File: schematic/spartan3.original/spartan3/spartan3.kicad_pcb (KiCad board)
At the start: 2 copper layers, 214.6 x 160 mm, 240 parts, among them U1_clk_select_0 SPFT_Sliding_Switch-dynacore, U2 XC3S250E-4TQG144C

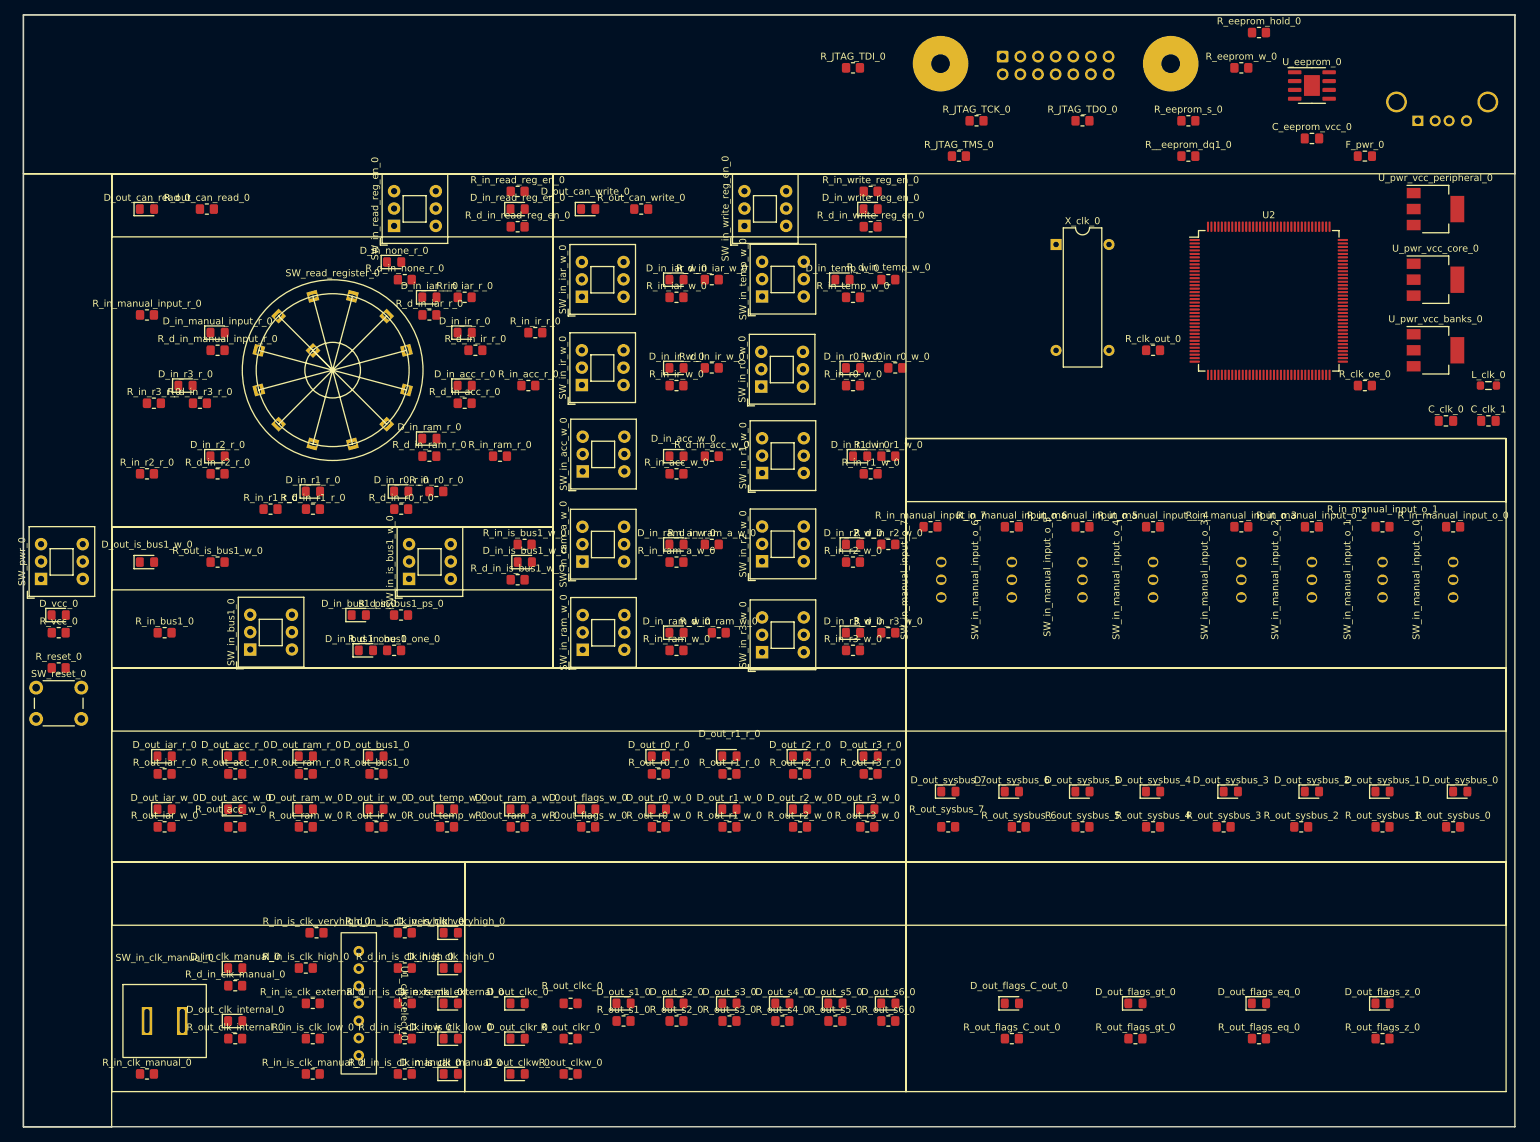
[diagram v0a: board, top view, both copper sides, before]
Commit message: PCB layout :: updated
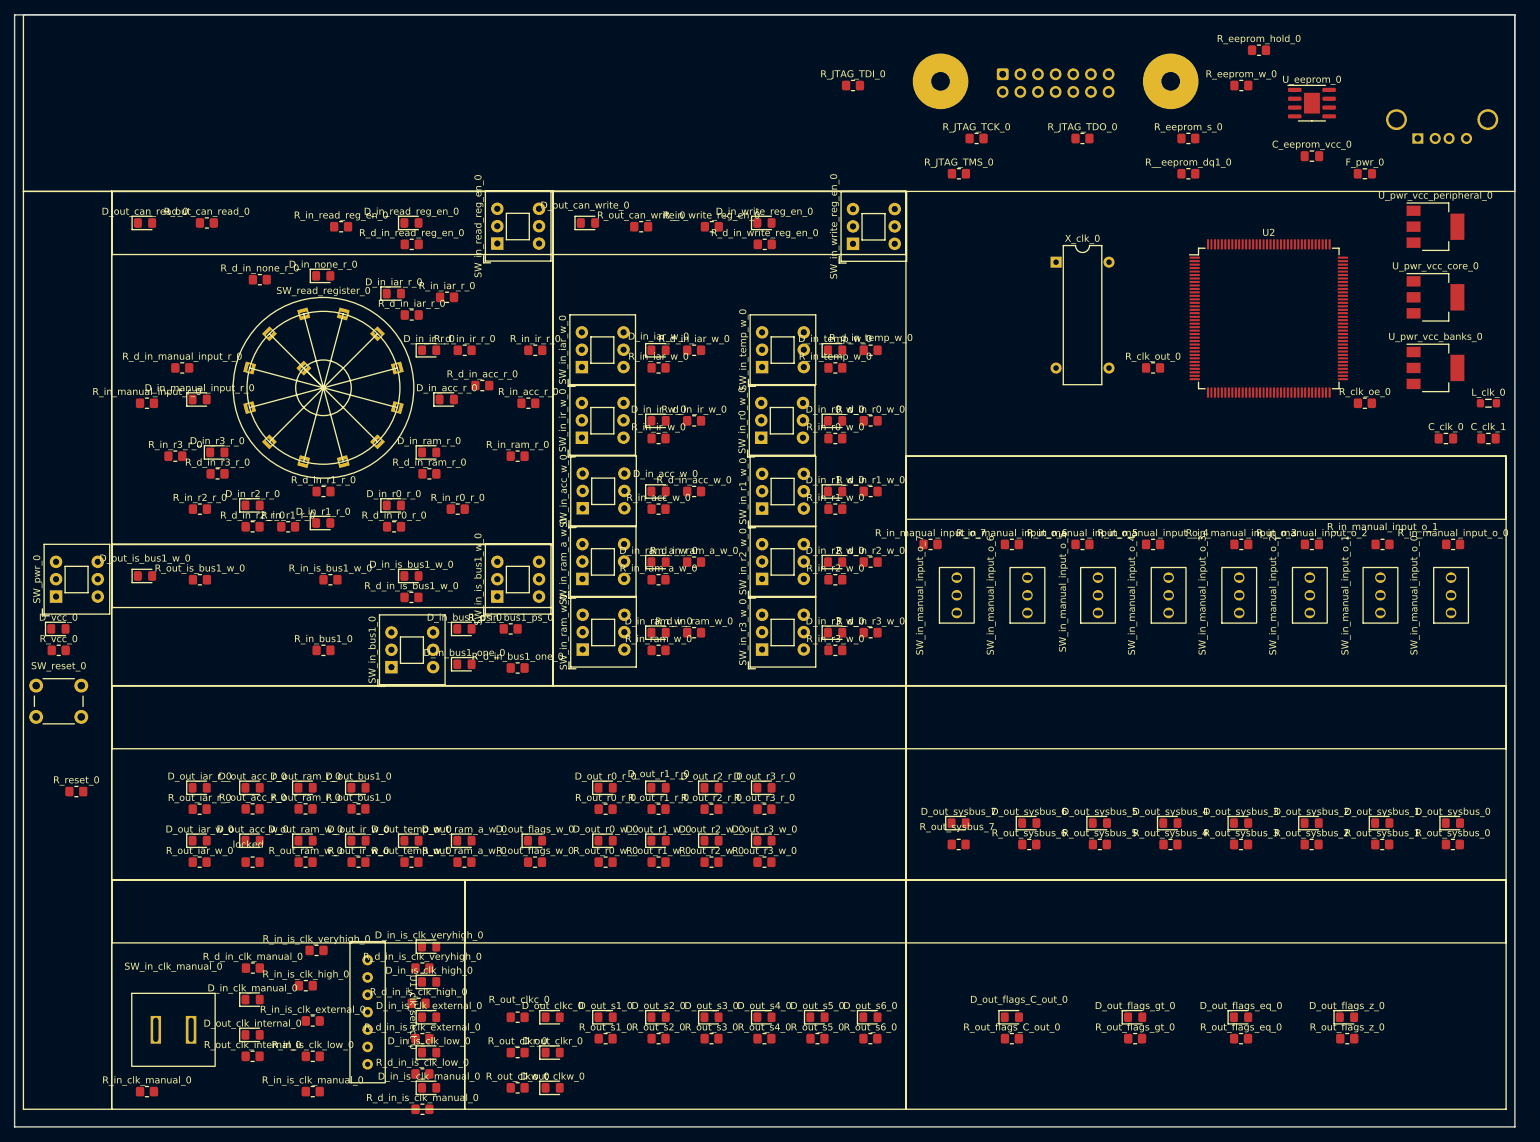
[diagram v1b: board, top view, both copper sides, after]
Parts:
- moved R_in_is_bus1_w_0 28.4 mm to (44.2, 81.3)
- moved R_in_read_reg_en_0 25.9 mm to (45.7, 30.5)
- moved R_in_write_reg_en_0 23.4 mm to (99.1, 30.5)
- moved R_in_bus1_0 23.0 mm to (43.2, 91.4)
- moved R_d_in_none_r_0 20.9 mm to (34.0, 38.1)
- moved SW_in_bus1_0 20.5 mm to (53.0, 93.9)
- moved R_d_in_bus1_one_0 18.0 mm to (71.1, 94.0)
- moved R_reset_0 18.0 mm to (7.62, 111.8)
- moved D_in_is_bus1_w_0 16.4 mm to (55.8, 80.7)
- moved R_out_r3_r_0 16.1 mm to (106.6, 114.3)
- moved D_out_r3_r_0 15.9 mm to (106.6, 111.2)
- moved R_d_in_bus1_ps_0 15.9 mm to (70.1, 88.4)
- moved SW_in_write_reg_en_0 15.8 mm to (119.4, 32.9)
- moved R_out_r3_w_0 15.6 mm to (106.6, 121.9)
- moved R_d_in_is_bus1_w_0 15.5 mm to (55.8, 83.8)
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- renumbered R_out_acc_w_0 to locked
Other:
- board size 214.6 x 160 mm -> 215.9 x 160 mm
